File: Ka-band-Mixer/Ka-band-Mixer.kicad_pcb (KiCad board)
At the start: 4 copper layers, 58.9 x 41.9 mm, 76 parts, among them J1 Conn_01x02_Male, J2 Conn_01x02_Male, J3 Connector_Conn_01x02_Male, J4 Conn_01x05_Male, J5 SMA_END-frequencySintesizer, U1 ADF4150HV, U2 LT1962-3.3, U3 LT3010, U4 HMC739LP4E, U5 LT1962-5, U6 LT1962-5, U7 HMC292ALC3B, X1 IQXT-220-1

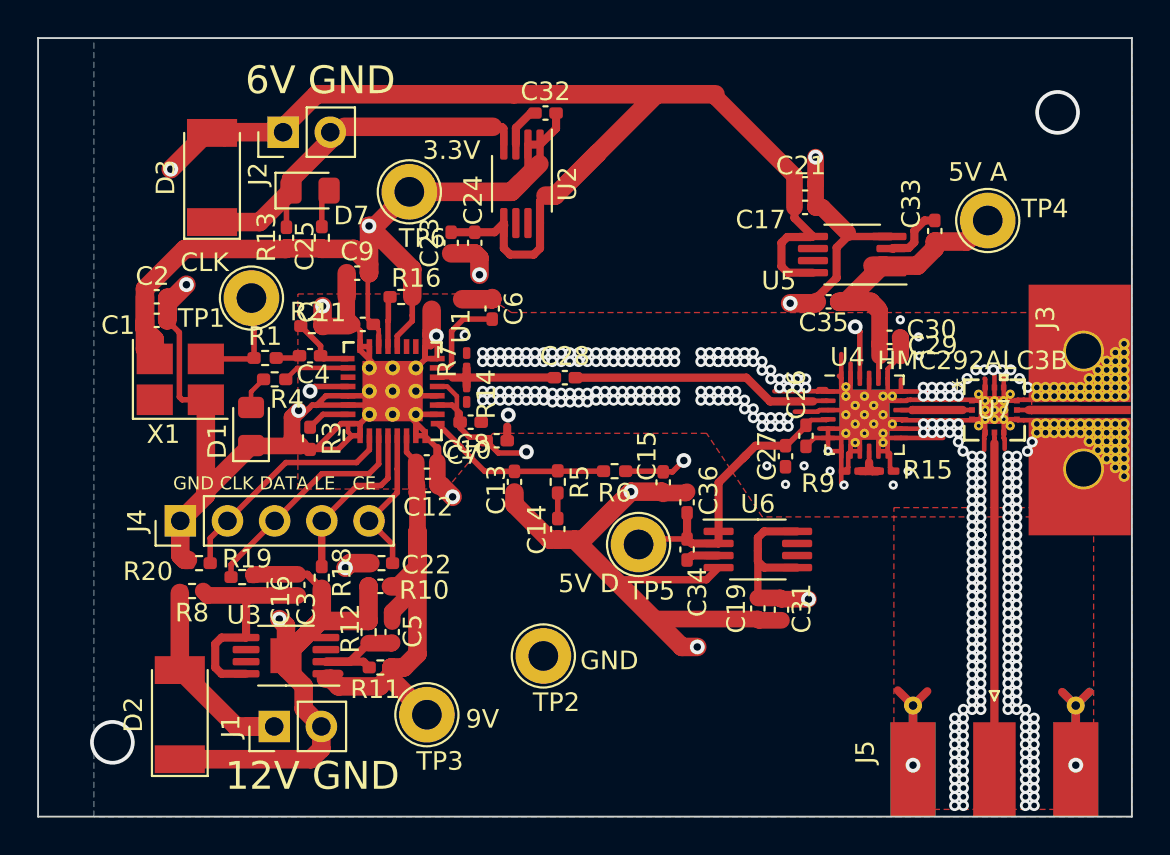
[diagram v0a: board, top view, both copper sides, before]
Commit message: some_update
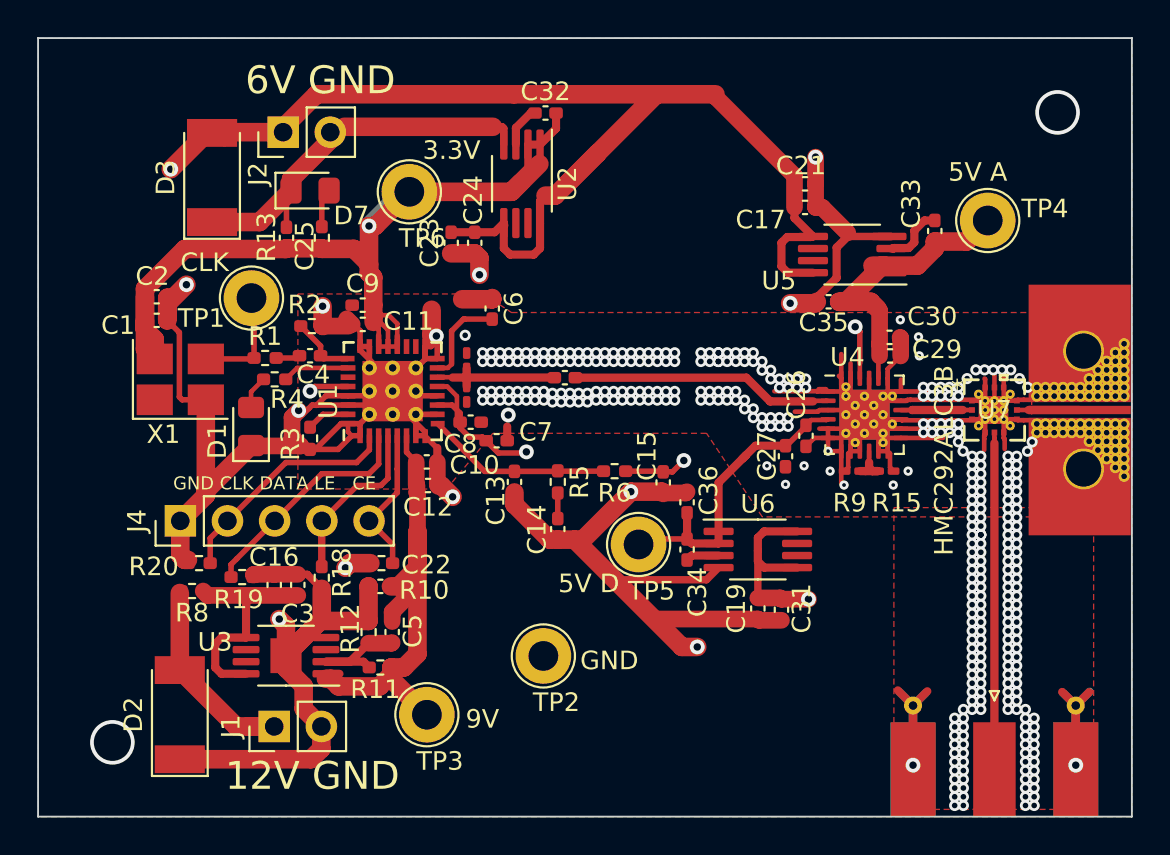
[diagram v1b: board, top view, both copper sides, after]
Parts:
- removed R16: 0, Resistor_SMD:R_0402_1005Metric_Pad0.72x0.64mm_HandSolder
- moved C9 1.75 mm to (106.7, 94.3)
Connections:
- U1 pad 21: Net-(R16-Pad2) -> +3V3
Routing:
- net Net-(R16-Pad2): track 2.74 -> 0.00 mm
- net 0: track 302.8 -> 300.4 mm
- net +3V3: track 128.3 -> 129.4 mm
